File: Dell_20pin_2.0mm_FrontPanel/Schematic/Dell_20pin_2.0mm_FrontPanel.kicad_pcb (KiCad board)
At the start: 2 copper layers, 36.8 x 14.5 mm, 6 parts, among them J1 DELL_2MM_MB_CONNECTOR, J2 HDD_LED_HEADER, J3 Conn_01x04, J4 HDAUDIO_HEADER, J5 Conn_01x05

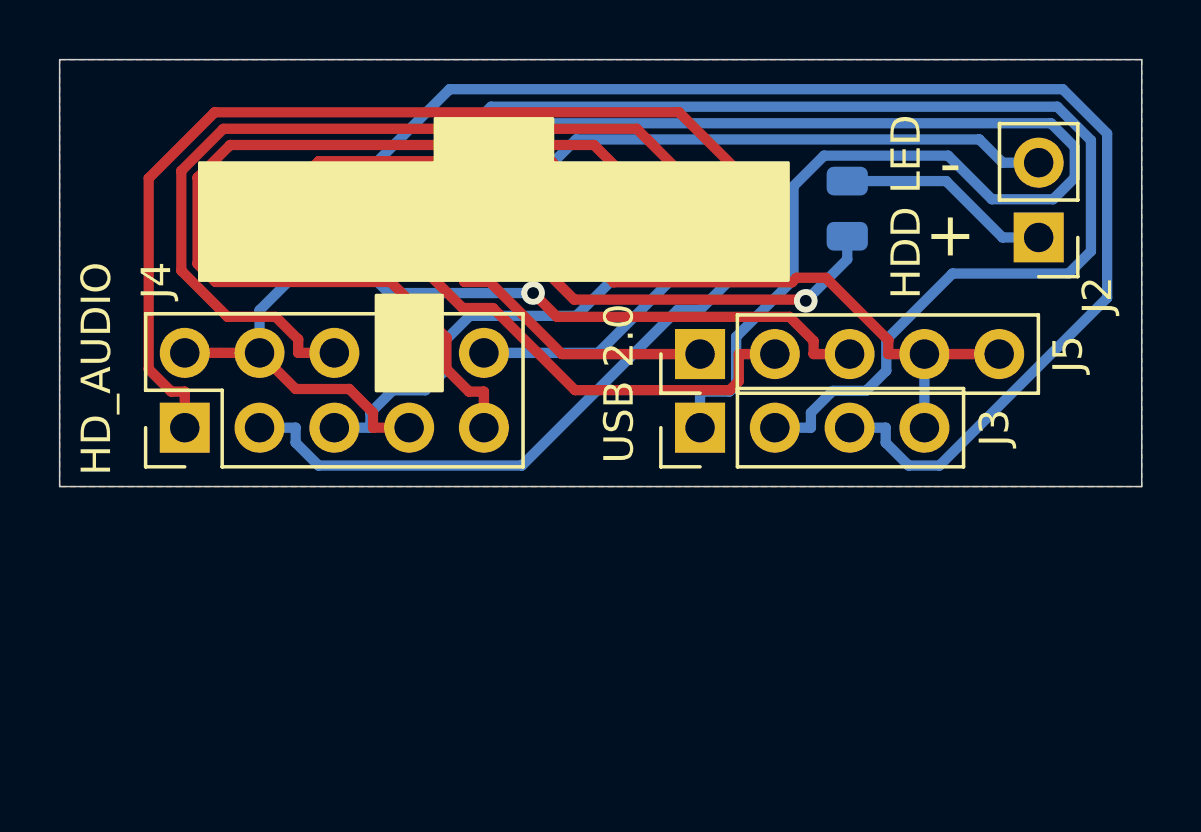
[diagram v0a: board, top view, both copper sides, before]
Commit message: start new PCB design
For some reason, when I load the original one in
pcbnew, it does not show any tracks, but also does
any rats nest connections.
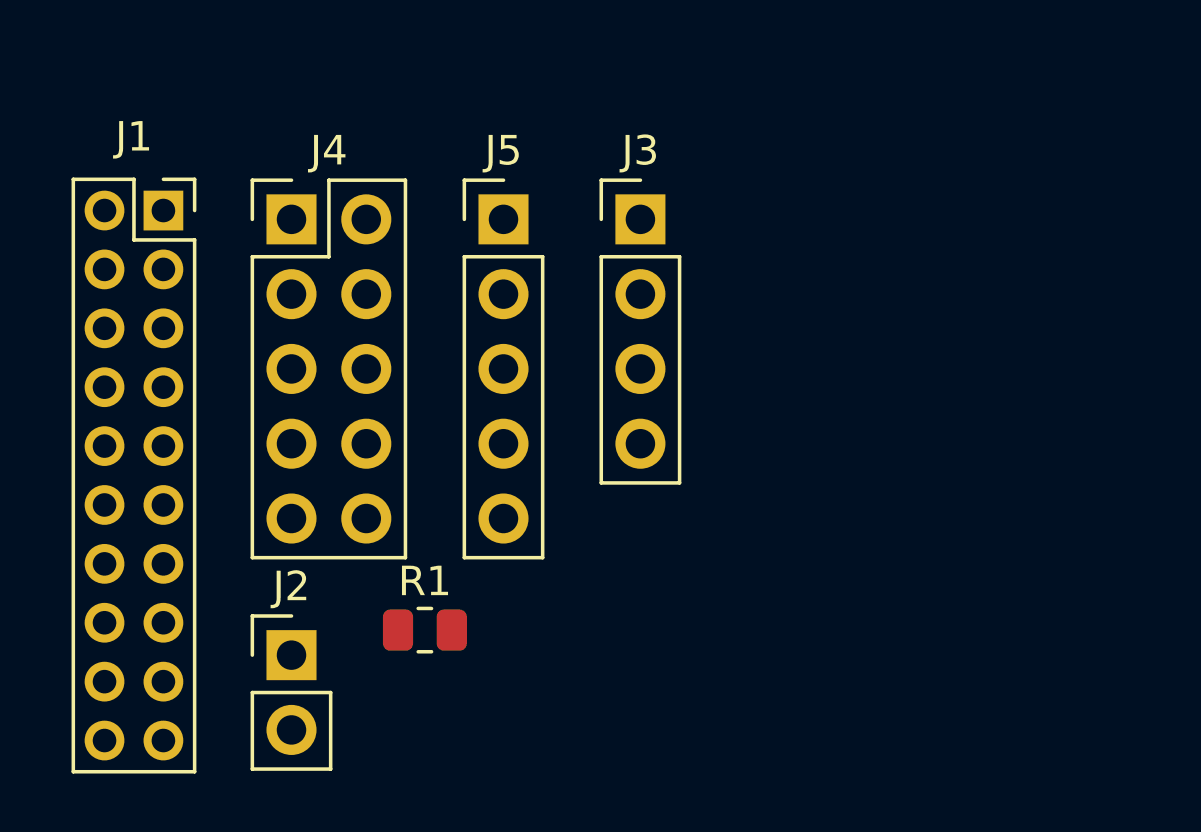
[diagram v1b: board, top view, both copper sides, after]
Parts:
- J1, R1: moved to F.Cu
- moved J2 29.1 mm to (146.9, 109.2), turned to 0 degrees
- moved R1 20.3 mm to (151.4, 108.4), turned to 0 degrees
- moved J1 20.2 mm to (142.5, 94.1), turned to 0 degrees
- moved J5 8.09 mm to (154.1, 94.4), turned to 0 degrees
- moved J4 7.95 mm to (146.9, 94.4), turned to 0 degrees
- moved J3 7.36 mm to (158.7, 94.4), turned to 0 degrees
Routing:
- net FRONT_IO_DET: track 48.2 -> 0.00 mm
- net USB_D+_1: track 45.4 -> 0.00 mm
- net USB_VCC1: track 44.1 -> 0.00 mm
- net USB_D-_1: track 42.8 -> 0.00 mm
- net HEADPHONE_L: track 32.5 -> 0.00 mm
- net MIC_L: track 32.0 -> 0.00 mm
- net MIC_DET: track 29.1 -> 0.00 mm
- net MIC_R: track 20.8 -> 0.00 mm
- net USB_D+_2: track 18.8 -> 0.00 mm, vias 1 -> 0
- net HDD_LED-: track 18.6 -> 0.00 mm
- net USB_D-_2: track 15.5 -> 0.00 mm
- net HEADPHONE_R: track 13.8 -> 0.00 mm
- net HDD_LED+: track 13.1 -> 0.00 mm, vias 1 -> 0
- net USB_VCC2: track 10.1 -> 0.00 mm
- net HEADPHONE_DET: track 8.77 -> 0.00 mm
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- removed copper zone on B.Cu, net FRONT_IO_DET
- removed copper zone on F.Cu, net FRONT_IO_DET
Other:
- board outline removed
- net class Default: trace_width 0.35 -> 0.25
- board text removed: "- +"
- board text removed: "HDD LED"
- board text removed: "HD_AUDIO"
- board text removed: "Motherboard Side"
- board text removed: "OPTIPLEX 7010 7020 9010 9020 FP ADAPTER"
- board text removed: "USB 2.0"
- board text removed: "github.com/ harbinrepairs"
